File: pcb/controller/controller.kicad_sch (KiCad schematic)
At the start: 38 parts, among them J1 USB_B, J2 ISP, J3 AudioJack3, J4 Keys, SW17 Function, U2 ATtiny861A

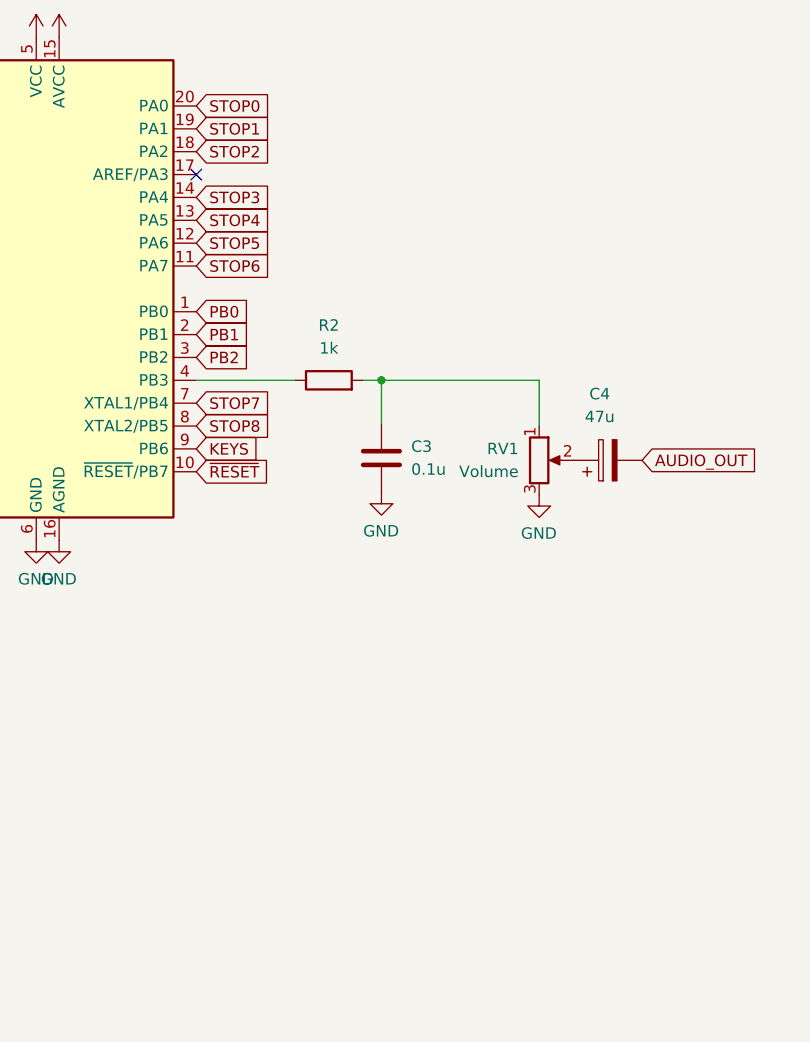
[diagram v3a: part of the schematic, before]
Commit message: Save
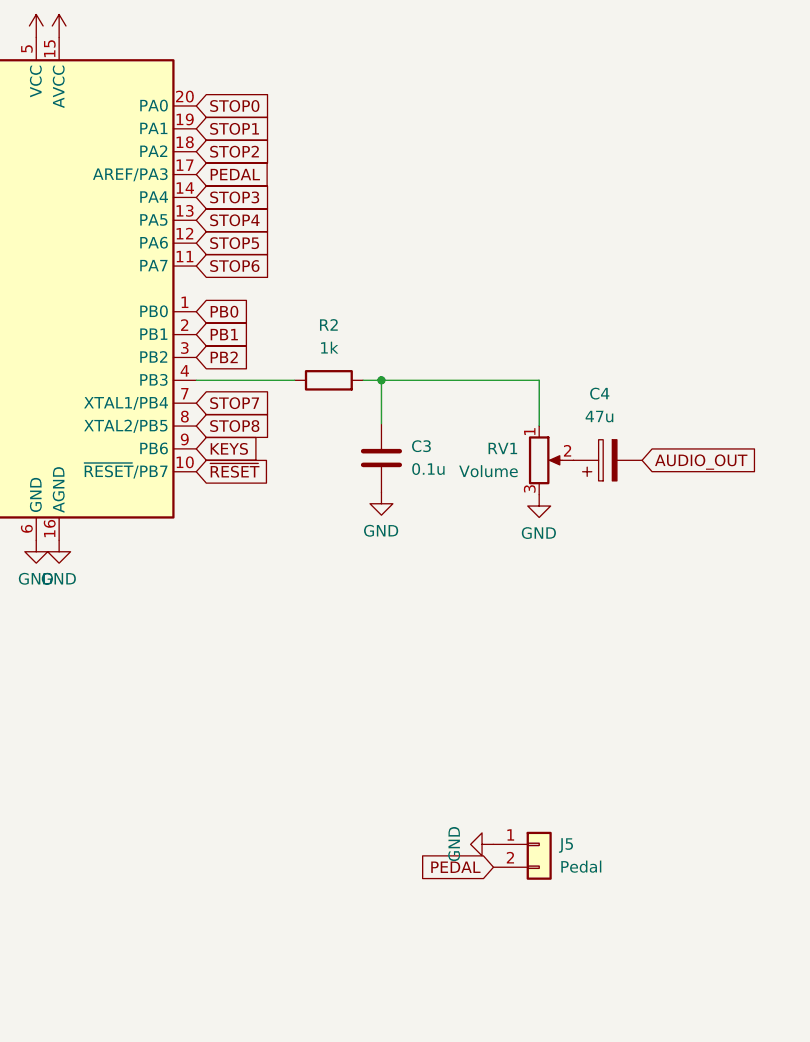
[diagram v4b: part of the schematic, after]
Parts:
- added J5: Pedal, Connector_PinHeader_2.54mm:PinHeader_1x02_P2.54mm_Vertical, symbol Connector_Generic:Conn_01x02
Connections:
- net GND: now also J5.1 (Pin_1)
- net PEDAL: now reaches U2.17 (AREF/PA3)
- net PEDAL: now also J5.2 (Pin_2)
- no-connect marks 3 -> 2
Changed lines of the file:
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@@
   (junction (at 224.028 60.706) (diameter 0) (color 0 0 0 0)
   )
-  (no_connect (at 203.454 37.846))
   (no_connect (at 44.704 37.084))
   (no_connect (at 44.704 34.544))
@@
     )
   )
+  (global_label "PEDAL" (shape input) (at 203.454 37.846 0) (fields_autoplaced)
+    (effects (font (size 1.27 1.27)) (justify left))
+    (property "Intersheet References" "${INTERSHEET_REFS}" (id 0) (at 211.6728 37.7666 0)
+      (effects (font (size 1.27 1.27)) (justify left) hide)
+    )
+  )
   (global_label "STOP3" (shape input) (at 103.632 112.776 0) (fields_autoplaced)
     (effects (font (size 1.27 1.27)) (justify left))
@@
     (property "Intersheet References" "${INTERSHEET_REFS}" (id 0) (at 211.8542 32.6866 0)
       (effects (font (size 1.27 1.27)) (justify left) hide)
+    )
+  )
+  (global_label "PEDAL" (shape input) (at 236.474 114.808 180) (fields_autoplaced)
+    (effects (font (size 1.27 1.27)) (justify right))
+    (property "Intersheet References" "${INTERSHEET_REFS}" (id 0) (at 228.2552 114.8874 0)
+      (effects (font (size 1.27 1.27)) (justify right) hide)
     )
   )
@@
     (pin "2")
   )
+  (symbol (lib_id "power:GND") (at 236.474 112.268 270) (unit 1)
+    (in_bom yes) (on_board yes)
+    (property "Reference" "#PWR0107" (id 0) (at 230.124 112.268 0)
+      (effects (font (size 1.27 1.27)) hide)
+    )
+    (property "Value" "GND" (id 1) (at 232.156 110.236 0)
+      (effects (font (size 1.27 1.27)) (justify left))
+    )
+    (property "Footprint" "" (id 2) (at 236.474 112.268 0)
+      (effects (font (size 1.27 1.27)) hide)
+    )
+    (property "Datasheet" "" (id 3) (at 236.474 112.268 0)
+      (effects (font (size 1.27 1.27)) hide)
+    )
+    (pin "1")
+  )
   (symbol (lib_id "power:VCC") (at 148.59 107.95 0) (unit 1)
     (in_bom yes) (on_board yes) (fields_autoplaced)
@@
       (effects (font (size 1.27 1.27)) hide)
     )
+  )
+  (symbol (lib_id "Connector_Generic:Conn_01x02") (at 241.554 112.268 0) (unit 1)
+    (in_bom yes) (on_board yes) (fields_autoplaced)
+    (property "Reference" "J5" (id 0) (at 243.84 112.2679 0)
+      (effects (font (size 1.27 1.27)) (justify left))
+    )
+    (property "Value" "Pedal" (id 1) (at 243.84 114.8079 0)
+      (effects (font (size 1.27 1.27)) (justify left))
+    )
+    (property "Footprint" "Connector_PinHeader_2.54mm:PinHeader_1x02_P2.54mm_Vertical" (id 2) (at 241.554 112.268 0)
+      (effects (font (size 1.27 1.27)) hide)
+    )
+    (property "Datasheet" "~" (id 3) (at 241.554 112.268 0)
+      (effects (font (size 1.27 1.27)) hide)
+    )
+    (pin "1")
+    (pin "2")
   )
   (symbol (lib_id "Device:R_Potentiometer") (at 78.994 112.776 0) (unit 1)
@@
       (reference "#PWR0106") (unit 1) (value "GND") (footprint "")
     )
+    (path "/dc2bc638-4dfc-4376-993e-ac519e38723e"
+      (reference "#PWR0107") (unit 1) (value "GND") (footprint "")
+    )
     (path "/b29902c5-8636-4234-87b8-7fcbad691fb8"
       (reference "#PWR0108") (unit 1) (value "VCC") (footprint "")
@@
       (reference "J4") (unit 1) (value "Keys") (footprint "Connector_PinHeader_2.54mm:PinHeader_1x06_P2.54mm_Vertical")
     )
+    (path "/f820df26-91ec-4248-80f8-a20a868197a0"
+      (reference "J5") (unit 1) (value "Pedal") (footprint "Connector_PinHeader_2.54mm:PinHeader_1x02_P2.54mm_Vertical")
+    )
     (path "/3a259560-8afb-487f-9ccd-4e59c4462820"

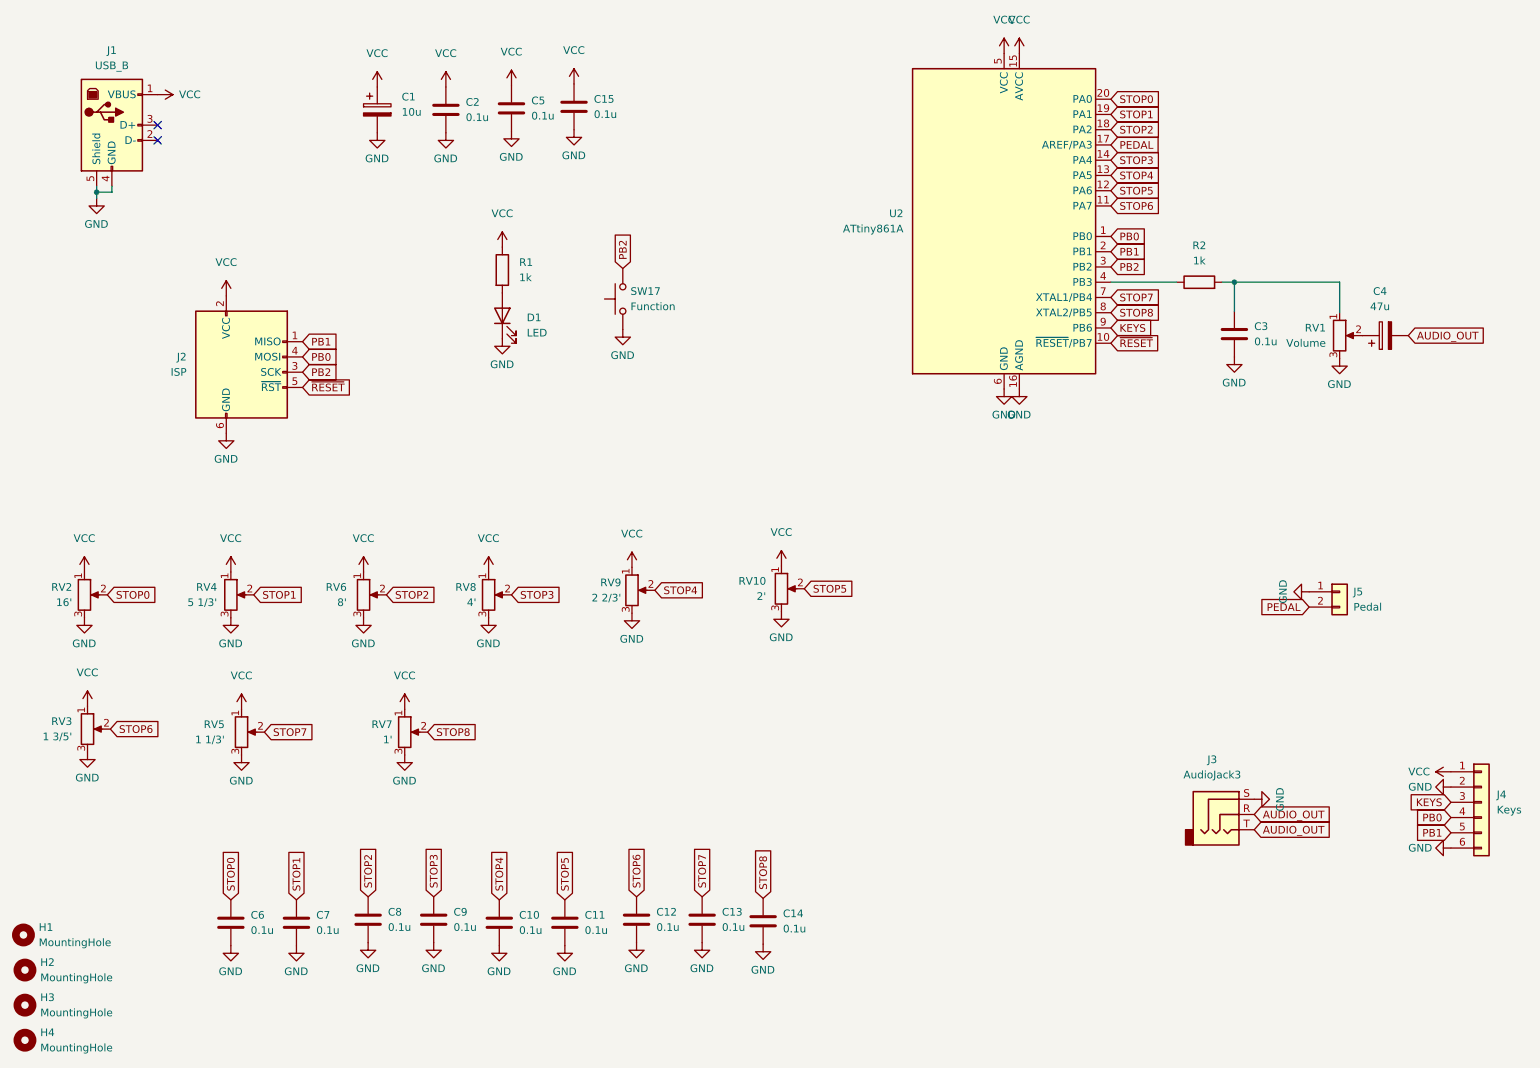
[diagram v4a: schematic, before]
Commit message: Boards ordered.
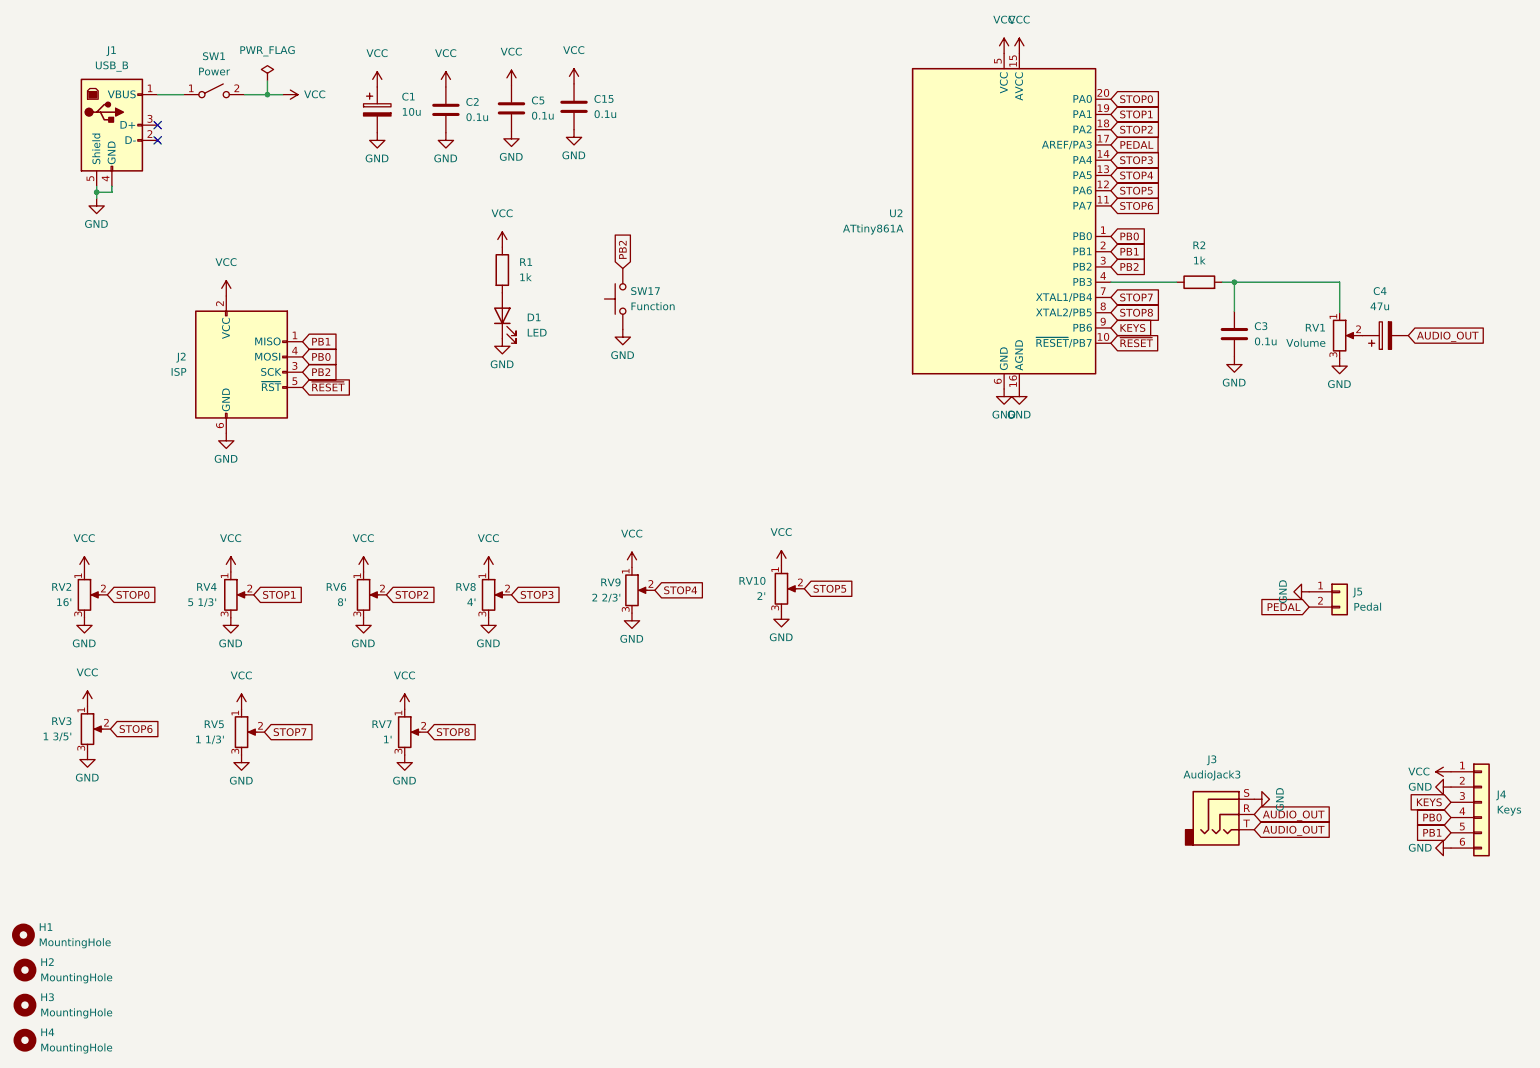
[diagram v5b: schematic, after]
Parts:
- removed C10, C11, C12, C13, C14, C6, C7, C8, C9: 0.1u, Capacitor_THT:C_Disc_D3.0mm_W2.0mm_P2.50mm, symbol Device:C
- added SW1: Power, Connector_PinHeader_2.54mm:PinHeader_1x03_P2.54mm_Vertical, symbol Switch:SW_SPST
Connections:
- net VCC: now also SW1.2 (B); no longer J1.1 (VBUS)
- new net: J1.1 (VBUS), SW1.1 (A)
